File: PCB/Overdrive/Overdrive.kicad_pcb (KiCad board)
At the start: 2 copper layers, 100 x 68 mm, 66 parts, among them J1 Alimentación, J10 FS2, J11 FS3, J12 FS6, J13 FS4, J2 Entrada, J3 Salida, J4 LM1117_3.3V, J5 OVD, J6 PWM, J7 OUT, J8 ADC_in, J9 FS1, SW2 BT_sw, SW3 RotaryEncoder_Switch, U1 TL072, U2 TL072

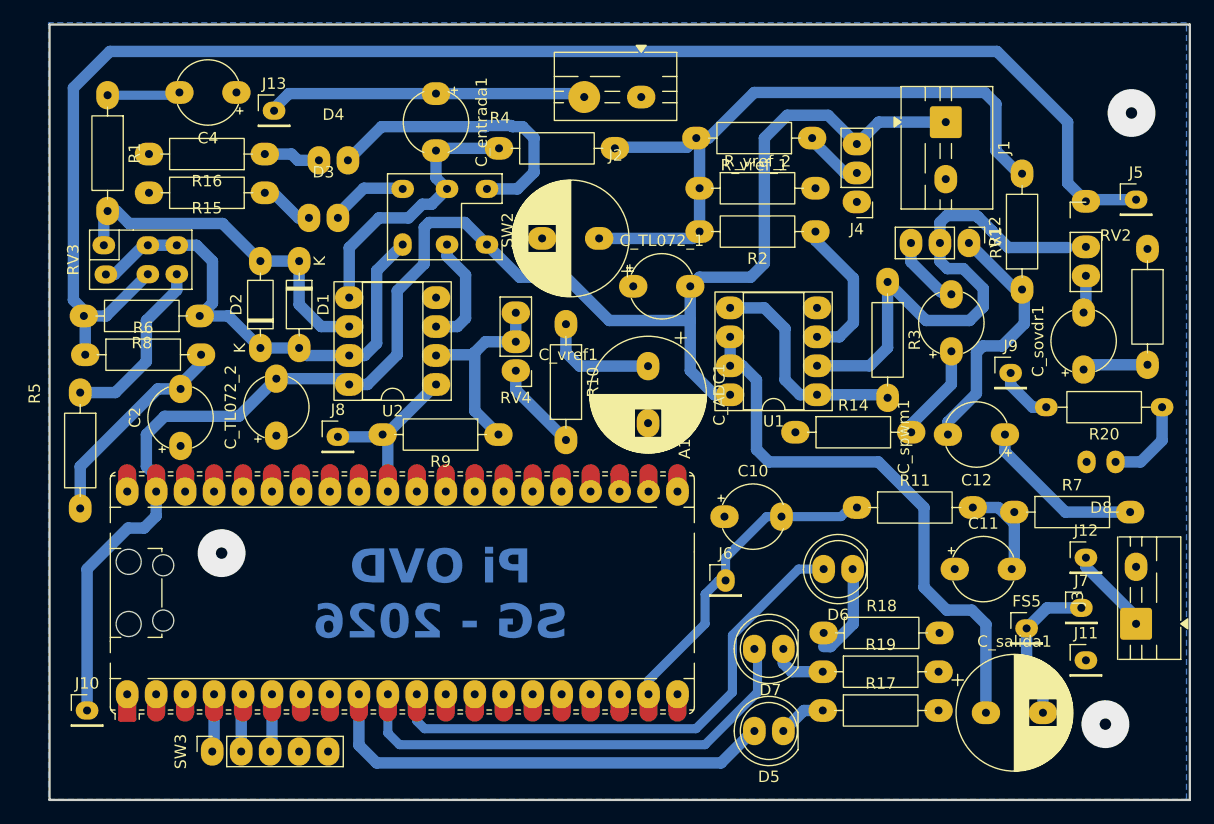
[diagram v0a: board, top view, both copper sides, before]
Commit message: A
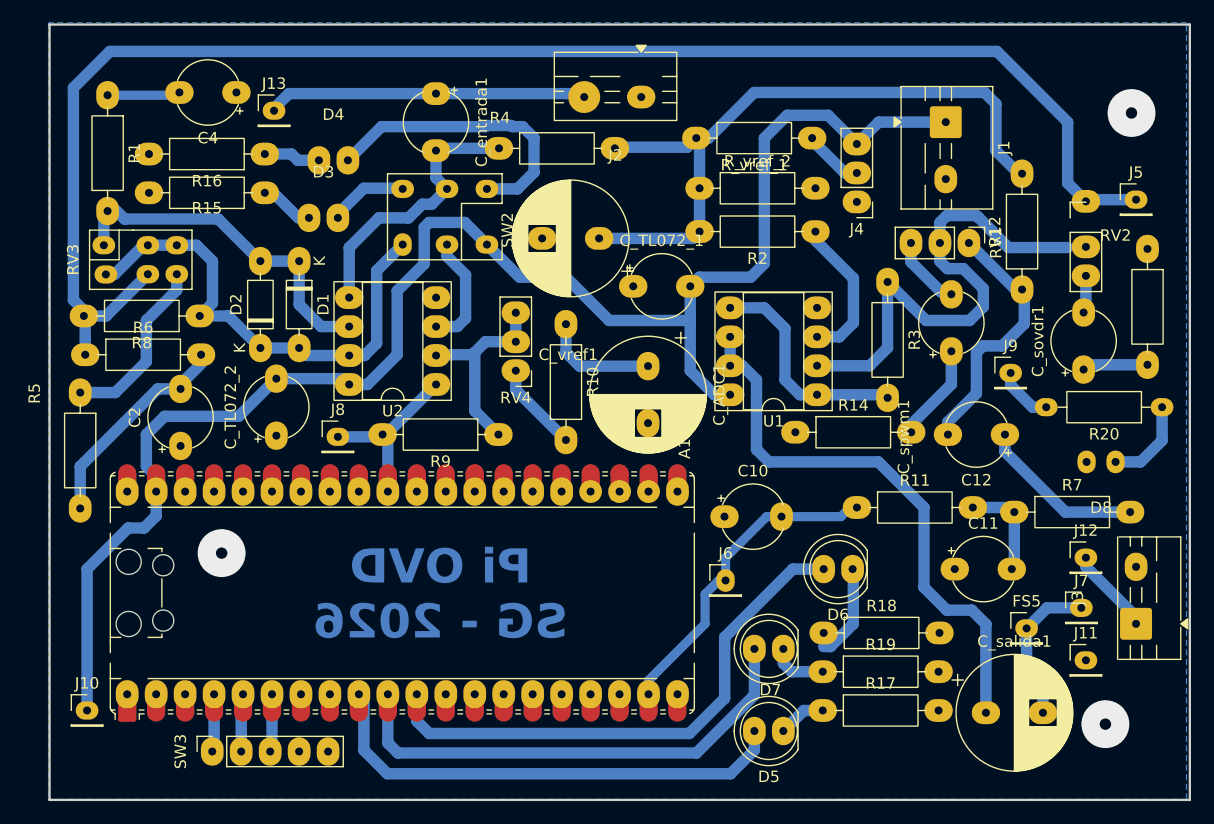
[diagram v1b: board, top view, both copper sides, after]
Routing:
- net Net-(A1-GPIO6): track 41.0 -> 42.7 mm
- net Net-(A1-GPIO7): track 42.1 -> 42.9 mm
- net Net-(C11-Pad2): track 8.44 -> 9.03 mm
- net Net-(A1-GPIO8): track 47.0 -> 47.6 mm
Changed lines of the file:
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@@
 		(sheetname "/")
 		(sheetfile "Overdrive.kicad_sch")
+		(units
+			(unit
+				(name "A")
+				(pins "1" "2")
+			)
+		)
 		(attr through_hole)
 		(duplicate_pad_numbers_are_jumpers no)
@@
 		(sheetname "/")
 		(sheetfile "Overdrive.kicad_sch")
+		(units
+			(unit
+				(name "A")
+				(pins "1" "2")
+			)
+		)
 		(attr through_hole)
 		(duplicate_pad_numbers_are_jumpers no)
@@
 		(sheetname "/")
 		(sheetfile "Overdrive.kicad_sch")
+		(units
+			(unit
+				(name "A")
+				(pins "1" "2")
+			)
+		)
 		(attr through_hole)
 		(duplicate_pad_numbers_are_jumpers no)
@@
 		(sheetname "/")
 		(sheetfile "Overdrive.kicad_sch")
+		(units
+			(unit
+				(name "A")
+				(pins "1" "2")
+			)
+		)
 		(attr through_hole)
 		(duplicate_pad_numbers_are_jumpers no)
@@
 	)
 	(segment
-		(start 47.69 133.29)
-		(end 50.99 136.59)
-		(width 1)
-		(layer "B.Cu")
-		(net "Net-(D1-K)")
-	)
-	(segment
-		(start 37.6 132.2)
-		(end 38.39 132.2)
+		(start 56.33 142.33)
+		(end 58.79 142.33)
 		(width 1)
 		(layer "B.Cu")
@@
 	)
 	(segment
-		(start 39.48 133.29)
-		(end 47.69 133.29)
+		(start 50.99 136.59)
+		(end 54.4 136.59)
 		(width 1)
 		(layer "B.Cu")
@@
 	)
 	(segment
-		(start 50.99 136.59)
-		(end 54.4 136.59)
+		(start 54.4 136.59)
+		(end 54.4 140.4)
 		(width 1)
 		(layer "B.Cu")
@@
 	)
 	(segment
-		(start 56.33 142.33)
-		(end 58.79 142.33)
+		(start 37.6 132.2)
+		(end 38.39 132.2)
 		(width 1)
 		(layer "B.Cu")
@@
 	)
 	(segment
-		(start 54.4 136.59)
-		(end 54.4 140.4)
+		(start 39.09 132.9)
+		(end 47.3 132.9)
 		(width 1)
 		(layer "B.Cu")
@@
 	)
 	(segment
+		(start 47.3 132.9)
+		(end 50.99 136.59)
+		(width 1)
+		(layer "B.Cu")
+		(net "Net-(D1-K)")
+	)
+	(segment
 		(start 38.39 132.2)
-		(end 39.48 133.29)
+		(end 39.09 132.9)
 		(width 1)
 		(layer "B.Cu")
@@
 	)
 	(segment
-		(start 61.2 180.6)
-		(end 91.4 180.6)
+		(start 94.325 179.465)
+		(end 94.325 177.8)
 		(width 1)
 		(layer "B.Cu")
@@
 	)
 	(segment
-		(start 93.985 178.14)
-		(end 94.325 177.8)
+		(start 59.64 174.58)
+		(end 60.08 175.02)
 		(width 1)
 		(layer "B.Cu")
@@
 	)
 	(segment
-		(start 91.4 180.6)
-		(end 93.86 178.14)
+		(start 62.15 181.55)
+		(end 92.24 181.55)
 		(width 1)
 		(layer "B.Cu")
@@
 	)
 	(segment
-		(start 59.64 179.04)
-		(end 61.2 180.6)
+		(start 60.08 179.48)
+		(end 62.15 181.55)
 		(width 1)
 		(layer "B.Cu")
@@
 	)
 	(segment
-		(start 59.64 174.58)
-		(end 59.64 179.04)
+		(start 60.08 175.02)
+		(end 60.08 179.48)
 		(width 1)
 		(layer "B.Cu")
@@
 	)
 	(segment
-		(start 93.86 178.14)
-		(end 93.985 178.14)
+		(start 92.24 181.55)
+		(end 94.325 179.465)
 		(width 1)
 		(layer "B.Cu")
@@
 	)
 	(segment
-		(start 90 179)
-		(end 94.6 174.4)
-		(width 0.8)
-		(layer "B.Cu")
-		(net "Net-(A1-GPIO7)")
-	)
-	(segment
-		(start 94.6 174.4)
-		(end 94.6 170.875)
-		(width 0.8)
+		(start 94.325 174.655)
+		(end 94.325 170.6)
+		(width 1)
 		(layer "B.Cu")
 		(net "Net-(A1-GPIO7)")
 	)
 	(segment
-		(start 94.6 170.875)
-		(end 94.325 170.6)
-		(width 0.8)
+		(start 62.18 174.58)
+		(end 62.18 178.85)
+		(width 1)
 		(layer "B.Cu")
 		(net "Net-(A1-GPIO7)")
 	)
 	(segment
-		(start 62.18 177.98)
-		(end 63.2 179)
-		(width 0.8)
+		(start 89.25 179.73)
+		(end 94.325 174.655)
+		(width 1)
 		(layer "B.Cu")
 		(net "Net-(A1-GPIO7)")
 	)
 	(segment
-		(start 63.2 179)
-		(end 90 179)
-		(width 0.8)
+		(start 63.06 179.73)
+		(end 89.25 179.73)
+		(width 1)
 		(layer "B.Cu")
 		(net "Net-(A1-GPIO7)")
 	)
 	(segment
-		(start 62.18 174.58)
-		(end 62.18 177.98)
-		(width 0.8)
+		(start 62.18 178.85)
+		(end 63.06 179.73)
+		(width 1)
 		(layer "B.Cu")
 		(net "Net-(A1-GPIO7)")
 	)
 	(segment
-		(start 92.4 169.4)
-		(end 92.4 174.4)
-		(width 0.8)
+		(start 64.72 176.93)
+		(end 65.81 178.02)
+		(width 1)
 		(layer "B.Cu")
 		(net "Net-(A1-GPIO8)")
 	)
 	(segment
-		(start 100.4 163.6)
-		(end 98.2 163.6)
-		(width 0.8)
+		(start 97.7 163.6)
+		(end 100.4 163.6)
+		(width 1)
 		(layer "B.Cu")
 		(net "Net-(A1-GPIO8)")
 	)
 	(segment
-		(start 89.2 177.6)
-		(end 65.4 177.6)
-		(width 0.8)
+		(start 65.81 178.02)
+		(end 88.63 178.02)
+		(width 1)
 		(layer "B.Cu")
 		(net "Net-(A1-GPIO8)")
 	)
 	(segment
-		(start 98.2 163.6)
-		(end 92.4 169.4)
-		(width 0.8)
+		(start 91.72 169.58)
+		(end 97.7 163.6)
+		(width 1)
 		(layer "B.Cu")
 		(net "Net-(A1-GPIO8)")
 	)
 	(segment
-		(start 92.4 174.4)
-		(end 89.2 177.6)
-		(width 0.8)
+		(start 88.63 178.02)
+		(end 91.72 174.93)
+		(width 1)
 		(layer "B.Cu")
 		(net "Net-(A1-GPIO8)")
 	)
 	(segment
-		(start 64.72 176.92)
-		(end 64.72 174.58)
-		(width 0.8)
+		(start 64.72 174.58)
+		(end 64.72 176.93)
+		(width 1)
 		(layer "B.Cu")
 		(net "Net-(A1-GPIO8)")
 	)
 	(segment
-		(start 65.4 177.6)
-		(end 64.72 176.92)
-		(width 0.8)
+		(start 91.72 174.93)
+		(end 91.72 169.58)
+		(width 1)
 		(layer "B.Cu")
 		(net "Net-(A1-GPIO8)")
@@
 	)
 	(segment
-		(start 113.48 158.2)
-		(end 115.72 158.2)
+		(start 116.72 158.2)
+		(end 117.12 158.6)
 		(width 1)
 		(layer "B.Cu")
@@
 	)
 	(segment
-		(start 115.72 158.2)
-		(end 117.12 159.6)
+		(start 113.48 158.2)
+		(end 116.72 158.2)
 		(width 1)
 		(layer "B.Cu")
@@
 	)
 	(segment
-		(start 117.12 159.6)
+		(start 117.12 158.6)
 		(end 117.12 163.82)
 		(width 1)
